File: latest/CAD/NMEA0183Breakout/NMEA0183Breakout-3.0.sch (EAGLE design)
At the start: 35 parts, among them IC1 LD2985BM50R, J1 10118194-0001LF, J2 RJ-82A86MMNL, Q1 DMP3099L-7, Q2 DMP3099L-7, Q3 DMP3099L-7, Q4 BSS138, U1 DS8921M

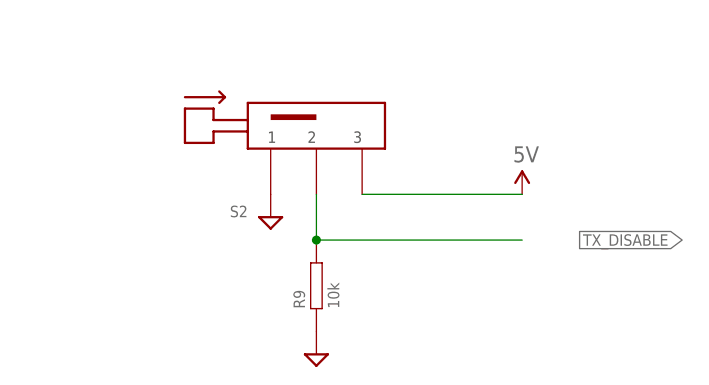
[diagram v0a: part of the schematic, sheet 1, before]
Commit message: Updated CAD
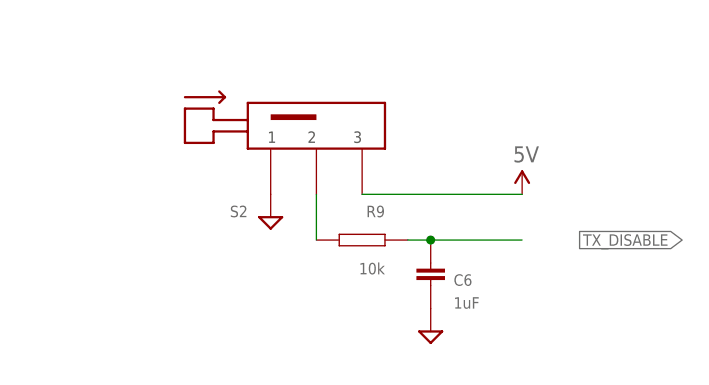
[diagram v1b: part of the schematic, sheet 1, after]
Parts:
- added C6: 1uF, MyPassives:CAPACITOR0603
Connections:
- new net N$5: R9.P$2, S2.2
- net GND: now also C6.2; no longer R9.P$1
- net TX_DISABLE: now also C6.1, R9.P$1; no longer R9.P$2, S2.2
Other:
- moved on the sheet: R9
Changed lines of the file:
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@@
 </attributes>
 <variantdefs>
-<variantdef name="NMEA0183" current="yes"/>
+<variantdef name="NMEA0183"/>
 </variantdefs>
 <classes>
@@
 <part name="SUPPLY22" library="SparkFun-Aesthetics" deviceset="5V" device=""/>
 <part name="R9" library="MyPassives" deviceset="RESISTOR" device="0603" value="10k"/>
-<part name="SUPPLY30" library="supply2" deviceset="GND" device=""/>
 <part name="R10" library="MyPassives" deviceset="RESISTOR" device="0603" value="10k"/>
 <part name="SUPPLY31" library="supply2" deviceset="GND" device=""/>
 <part name="SUPPLY26" library="supply2" deviceset="GND" device=""/>
 <part name="SUPPLY27" library="supply2" deviceset="GND" device=""/>
+<part name="C6" library="MyPassives" deviceset="CAPACITOR" device="0603" value="1uF"/>
+<part name="SUPPLY30" library="supply2" deviceset="GND" device=""/>
 </parts>
 <sheets>
@@
 <attribute name="VALUE" x="179.324" y="54.356" size="1.778" layer="96"/>
 </instance>
-<instance part="R9" gate="G$1" x="157.48" y="40.64" smashed="yes" rot="R90">
-<attribute name="NAME" x="156.21" y="38.1" size="1.27" layer="95" rot="R90"/>
-<attribute name="VALUE" x="160.02" y="38.1" size="1.27" layer="96" rot="R90"/>
-</instance>
-<instance part="SUPPLY30" gate="GND" x="157.48" y="33.02" smashed="yes"/>
+<instance part="R9" gate="G$1" x="162.56" y="45.72" smashed="yes" rot="R180">
+<attribute name="NAME" x="165.1" y="49.53" size="1.27" layer="95" rot="R180"/>
+<attribute name="VALUE" x="165.1" y="43.18" size="1.27" layer="96" rot="R180"/>
+</instance>
 <instance part="R10" gate="G$1" x="157.48" y="83.82" smashed="yes" rot="R90">
 <attribute name="NAME" x="156.21" y="81.28" size="1.27" layer="95" rot="R90"/>
@@
 <instance part="SUPPLY26" gate="GND" x="152.4" y="48.26" smashed="yes"/>
 <instance part="SUPPLY27" gate="GND" x="152.4" y="91.44" smashed="yes"/>
+<instance part="C6" gate="G$1" x="170.18" y="43.18" smashed="yes">
+<attribute name="NAME" x="172.72" y="40.64" size="1.27" layer="95"/>
+<attribute name="VALUE" x="172.72" y="38.1" size="1.27" layer="96"/>
+</instance>
+<instance part="SUPPLY30" gate="GND" x="170.18" y="35.56" smashed="yes"/>
 </instances>
 <busses>
@@
 </segment>
 <segment>
-<pinref part="R9" gate="G$1" pin="P$1"/>
-<pinref part="SUPPLY30" gate="GND" pin="GND"/>
-</segment>
-<segment>
 <pinref part="R10" gate="G$1" pin="P$1"/>
 <pinref part="SUPPLY31" gate="GND" pin="GND"/>
@@
 <pinref part="S1" gate="G$1" pin="1"/>
 <pinref part="SUPPLY27" gate="GND" pin="GND"/>
+</segment>
+<segment>
+<pinref part="SUPPLY30" gate="GND" pin="GND"/>
+<pinref part="C6" gate="G$1" pin="2"/>
 </segment>
 </net>
@@
 </segment>
 <segment>
-<wire x1="157.48" y1="45.72" x2="180.34" y2="45.72" width="0.1524" layer="91"/>
 <label x="198.12" y="45.72" size="1.27" layer="95" rot="R180" xref="yes"/>
-<pinref part="R9" gate="G$1" pin="P$2"/>
-<pinref part="S2" gate="G$1" pin="2"/>
-<wire x1="157.48" y1="50.8" x2="157.48" y2="45.72" width="0.1524" layer="91"/>
-<junction x="157.48" y="45.72"/>
+<pinref part="R9" gate="G$1" pin="P$1"/>
+<wire x1="180.34" y1="45.72" x2="170.18" y2="45.72" width="0.1524" layer="91"/>
+<pinref part="C6" gate="G$1" pin="1"/>
+<wire x1="170.18" y1="45.72" x2="167.64" y2="45.72" width="0.1524" layer="91"/>
+<junction x="170.18" y="45.72"/>
 </segment>
 </net>
@@
 </segment>
 </net>
+<net name="N$5" class="0">
+<segment>
+<pinref part="R9" gate="G$1" pin="P$2"/>
+<pinref part="S2" gate="G$1" pin="2"/>
+<wire x1="157.48" y1="50.8" x2="157.48" y2="45.72" width="0.1524" layer="91"/>
+</segment>
+</net>
